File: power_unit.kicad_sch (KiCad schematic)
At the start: 48 parts, among them J1 ATX-20, U1 LM7905_TO220, X1 Power, X10 RTC Standby, X2 Address, X3 Data, X4 Mode, X5 Control, X6 Clock, X7 Power SW, X8 Reset SW, X9 Power LED

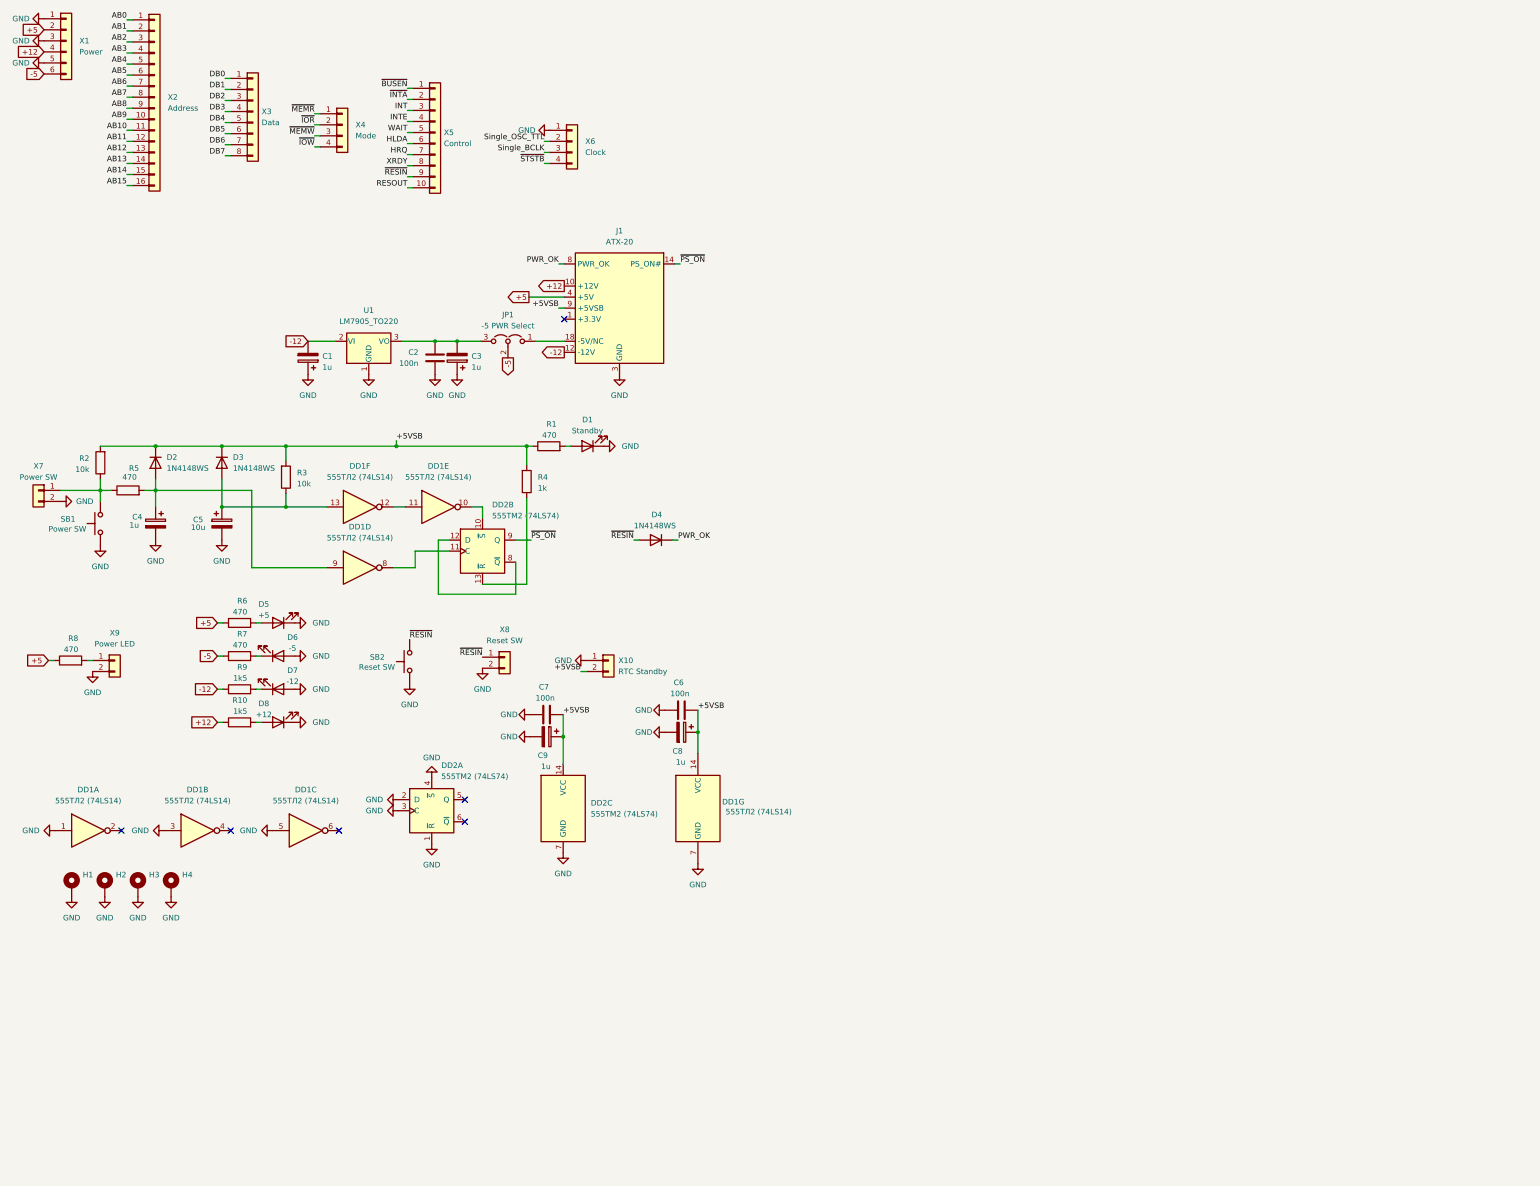
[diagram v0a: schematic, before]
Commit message: Update
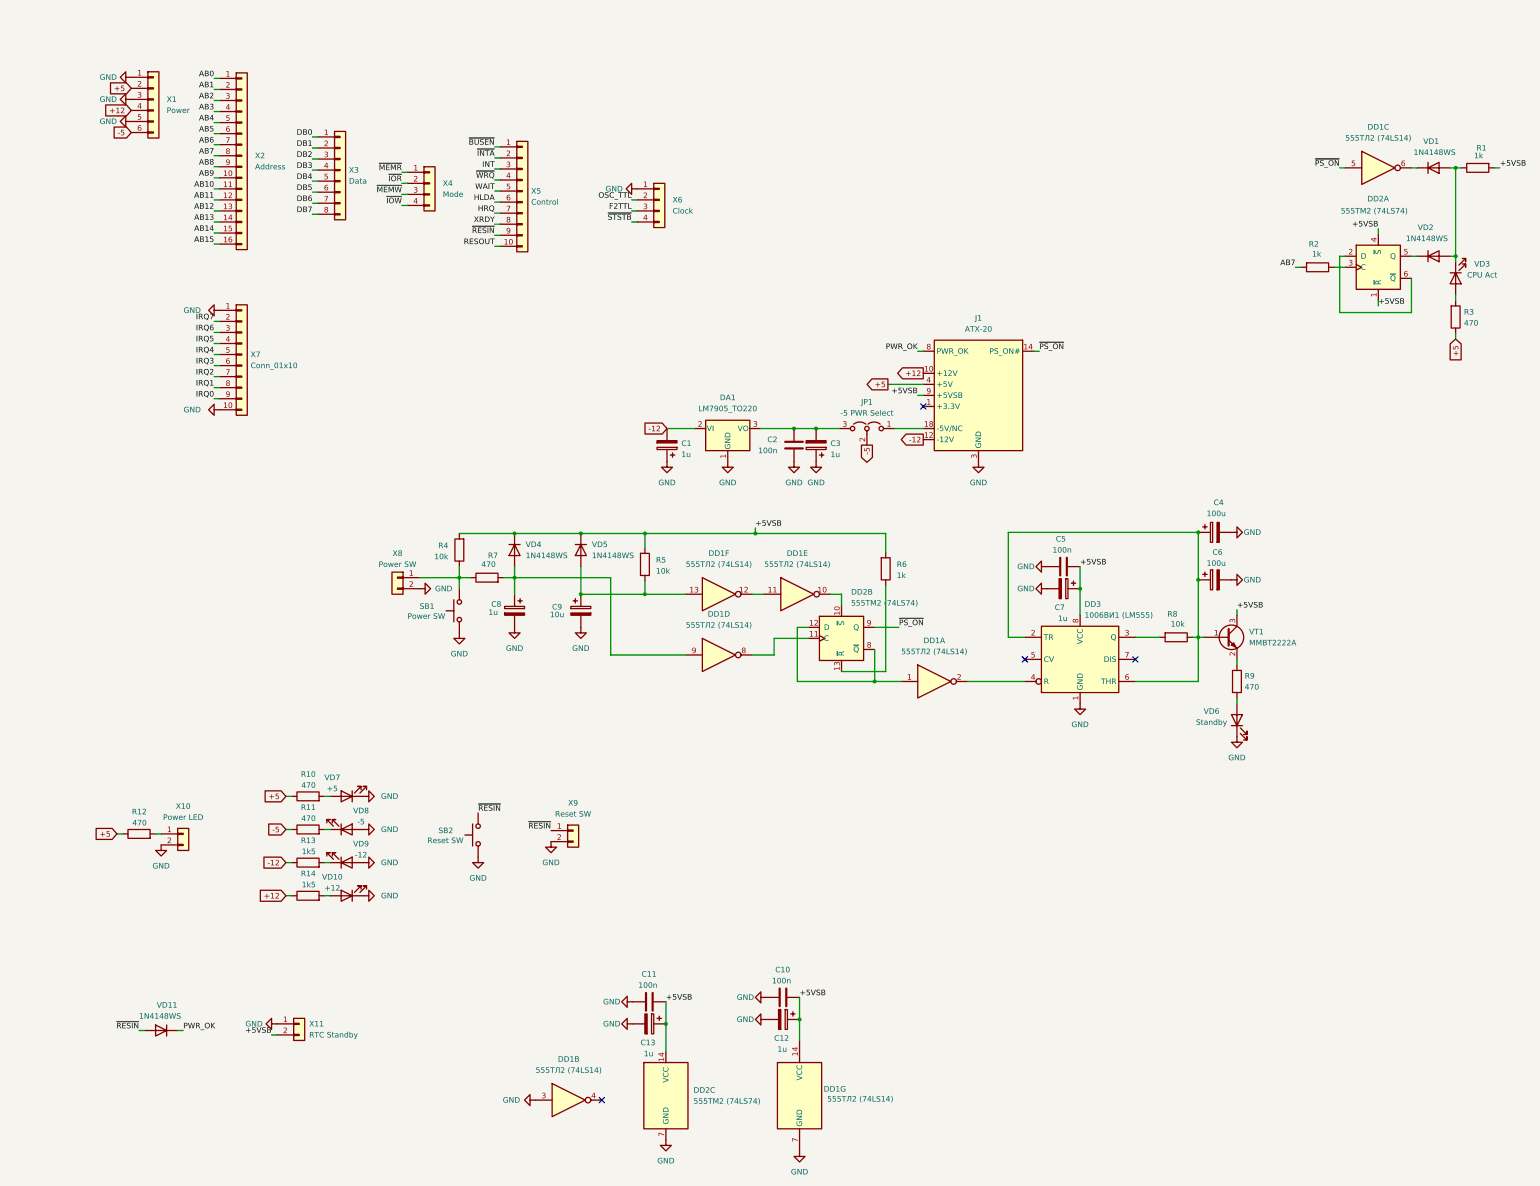
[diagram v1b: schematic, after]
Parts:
- removed H1, H2, H3, H4: MountingHole_Pad, MountingHole:MountingHole_3.2mm_M3_Pad_Via, symbol Mechanical:MountingHole_Pad
- added C4, C6: 100u, Capacitor_Tantalum_SMD:CP_EIA-3528-21_Kemet-B_Pad1.50x2.35mm_HandSolder, symbol Device:C_Polarized
- added C5: 100n, Capacitor_SMD:C_0805_2012Metric_Pad1.18x1.45mm_HandSolder, symbol Device:C
- added C7: 1u, Capacitor_Tantalum_SMD:CP_EIA-3216-18_Kemet-A_Pad1.58x1.35mm_HandSolder, symbol Device:C_Polarized
- added DD3: 1006ВИ1 (LM555), Package_DIP:DIP-8_W7.62mm_Socket_LongPads, symbol Timer:LM555xN
- added R1, R2: 1k, Resistor_SMD:R_0805_2012Metric_Pad1.20x1.40mm_HandSolder, symbol Device:R
- added R3: 470, Resistor_SMD:R_0805_2012Metric_Pad1.20x1.40mm_HandSolder, symbol Device:R
- added R8: 10k, Resistor_SMD:R_0805_2012Metric_Pad1.20x1.40mm_HandSolder, symbol Device:R
- added VD1, VD2: 1N4148WS, Diode_SMD:D_SOD-323_HandSoldering, symbol Diode:1N4148WS
- added VD3: CPU Act, LED_SMD:LED_0805_2012Metric_Pad1.15x1.40mm_HandSolder, symbol Device:LED
- added VT1: MMBT2222A, Package_TO_SOT_SMD:SOT-23_Handsoldering, symbol Transistor_BJT:MMBT2222A
- added X7: Conn_01x10, Connector_PinHeader_2.54mm:PinHeader_1x10_P2.54mm_Vertical, symbol Connector_Generic:Conn_01x10
- J1: footprint Connector_Molex:Molex_Mini-Fit_Jr_5566-20A2_2x10_P4.20mm_Vertical -> Library:ATX-20
- VD4: renamed from D2; footprint Diode_SMD:D_SOD-323 -> Diode_SMD:D_SOD-323_HandSoldering
- VD5: renamed from D3; footprint Diode_SMD:D_SOD-323 -> Diode_SMD:D_SOD-323_HandSoldering
- renumbered C6 to C10, C7 to C11, C8 to C12, C9 to C13, C4 to C8, C5 to C9, U1 to DA1, R6 to R10, R7 to R11, R8 to R12, R9 to R13, R10 to R14, R2 to R4, R3 to R5, R4 to R6, R5 to R7, R1 to R9, D8 to VD10, D4 to VD11, D1 to VD6, D5 to VD7, D6 to VD8, D7 to VD9, X9 to X10, X10 to X11, X7 to X8, X8 to X9
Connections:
- net +5: now also R3.1
- net +5VSB: now also DD2.1 (~{R}), DD2.4 (~{S}), C5.1, C7.1, DD3.8 (VCC), R1.2, VT1.3 (C); no longer R9.1
- net AB7: now also R2.2
- net GND: now also C4.2, C5.2, C6.2, C7.2, DD3.1 (GND), X7.1 (Pin_1), X7.10 (Pin_10); no longer DD1.1, DD1.5, DD2.1 (~{R}), DD2.2 (D), DD2.3 (C), DD2.4 (~{S})
- net ~{PS_ON}: now also DD1.5
- net at DD2.5 (Q): now also VD2.1 (K)
- net at DD2.6 (~{Q}): now also DD2.2 (D)
- net at DD1.2: now also DD3.4 (R)
- net at DD2.12 (D), DD2.8 (~{Q}): now also DD1.1
- net at DD1.6: now also VD1.1 (K)
- net INTE renamed ~{WRQ}
- net Single_BCLK renamed F2TTL
- net Single_OSC_TTL renamed OSC_TTL
- new net: R3.2, VD3.2 (A)
- new net: DD2.3 (C), R2.1
- new net: R9.1, VT1.2 (E)
- new net: C4.1, C6.1, DD3.2 (TR), DD3.6 (THR), R8.1, VT1.1 (B)
- new net: DD3.3 (Q), R8.2
- new net: R1.1, VD1.2 (A), VD2.2 (A), VD3.1 (K)
- new net IRQ0: X7.9 (Pin_9)
- new net IRQ1: X7.8 (Pin_8)
- new net IRQ2: X7.7 (Pin_7)
- new net IRQ3: X7.6 (Pin_6)
- new net IRQ4: X7.5 (Pin_5)
- new net IRQ5: X7.4 (Pin_4)
- new net IRQ6: X7.3 (Pin_3)
- new net IRQ7: X7.2 (Pin_2)
- no-connect marks 6 -> 4
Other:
- moved on the sheet: C1, C10, C11, C12, C13, C2, C3, C8, C9, DA1, DD1A, DD1B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
